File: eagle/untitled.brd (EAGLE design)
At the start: 56.8 x 71.1 mm, 30 parts, among them IC1 74HC595D, IC2 74HC595D, Q1 BC557, Q2 BC557, Q3 BC557, Q4 BC557, Q5 BC557, Q6 BC547, Q7 BC547, Q8 BC547

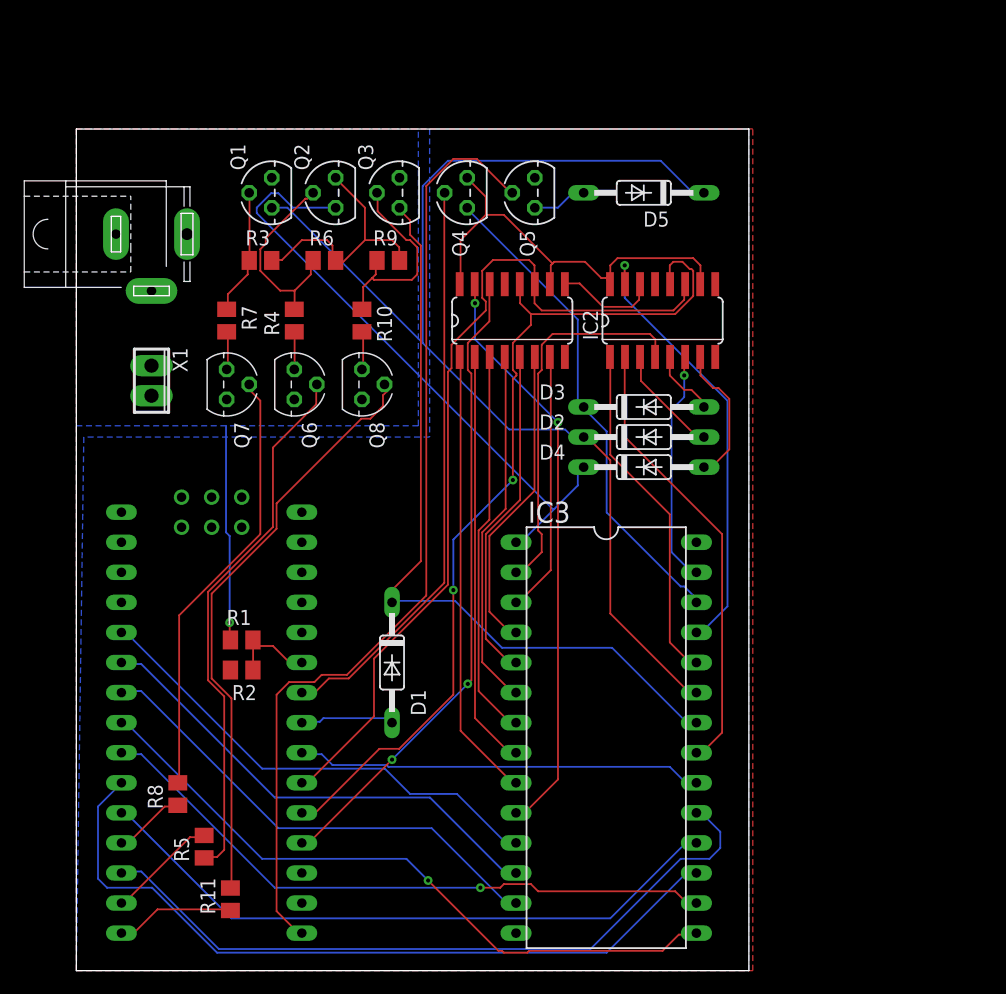
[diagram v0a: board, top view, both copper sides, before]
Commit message: Исправления схемы.
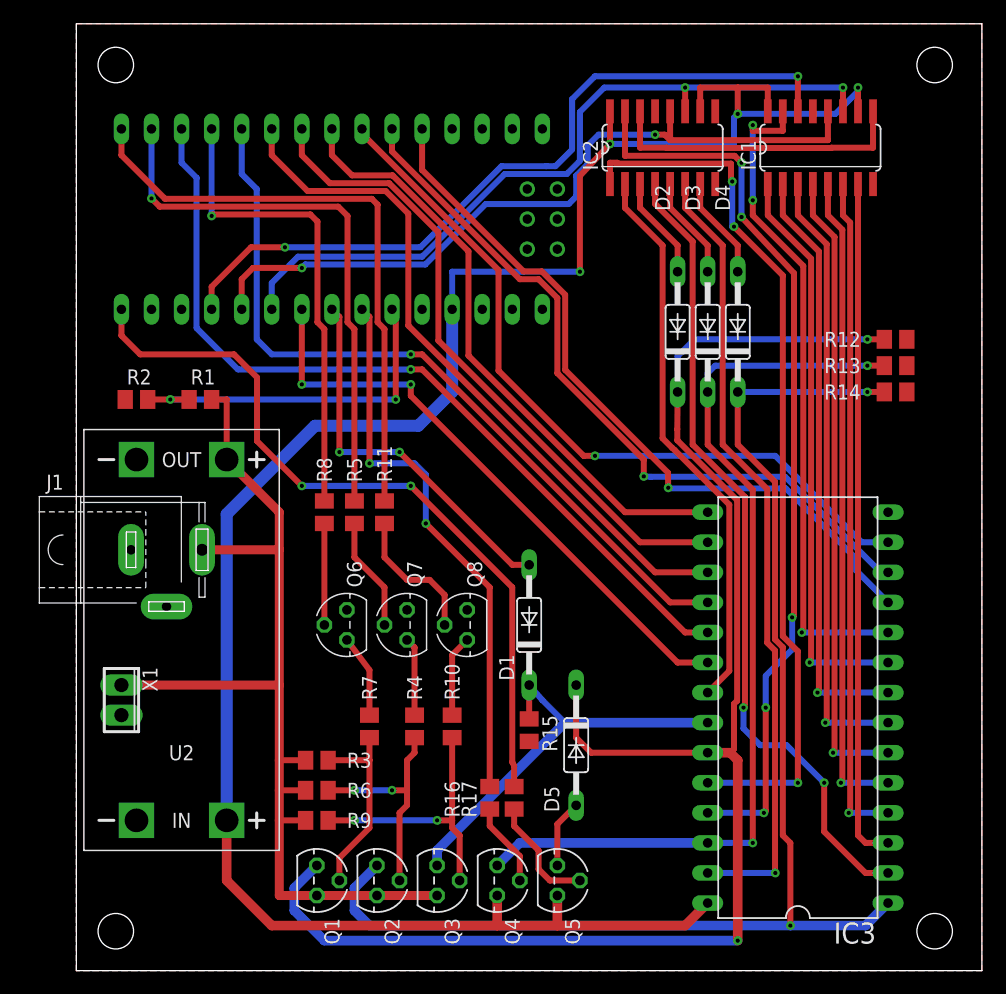
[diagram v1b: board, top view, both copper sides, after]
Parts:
- removed U$1: NANO, Arduino-clone:NANO
- added R12, R13, R14, R15: 4.7K, rcl:M0805
- added R16, R17: 300, rcl:M0805
- added U1: NANO, Arduino-clone:NANO
- added U2: DC-DC-STEP-UP-MT3608, diy-modules:DC-DC-STEP-UP-MT3608
- moved Q1 58.2 mm to (20.3, 7.62), turned to 270 degrees
- moved Q2 58.2 mm to (25.4, 7.62), turned to 270 degrees
- moved Q3 58.2 mm to (30.5, 7.62), turned to 270 degrees
- moved Q4 58.2 mm to (35.6, 7.62), turned to 270 degrees
- moved Q5 58.1 mm to (40.6, 7.62), turned to 270 degrees
- moved R9 47.7 mm to (20.3, 12.7), turned to 180 degrees
- moved D5 47.0 mm to (42.2, 19.1), turned to 270 degrees
- moved R6 44.8 mm to (20.3, 15.2), turned to 180 degrees
- moved R3 42.5 mm to (20.3, 17.8), turned to 180 degrees
- moved R7 36.4 mm to (24.8, 20.6), turned to 90 degrees
- moved R4 35.8 mm to (28.6, 20.6), turned to 270 degrees
- moved R11 35.2 mm to (26.0, 38.7), turned to 270 degrees
- moved R10 35.1 mm to (31.8, 20.6), turned to 90 degrees
- moved R5 31.0 mm to (23.5, 38.7)
- moved IC1 29.9 mm to (62.9, 69.5)
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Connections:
- new net N$25: Q4.2, R16.2
- new net N$26: Q5.2, R17.2
- net +24V: now also U2.OUT+
- net A11: now also R12.1
- net A13: now also R13.1
- net A15: now also R14.1
- net CE: now also U1.A3; no longer U$1.A3
- net D0: now also U1.D2; no longer U$1.D2
- net D1: now also U1.D3; no longer U$1.D3
- net D2: now also U1.D4; no longer U$1.D4
- net D3: now also U1.D5; no longer U$1.D5
- net D4: now also U1.D6; no longer U$1.D6
- net D5: now also U1.D7; no longer U$1.D7
- net D6: now also U1.D8; no longer U$1.D8
- net D7: now also U1.D10; no longer U$1.D10
- net GND: now also R12.2, R13.2, R14.2, R15.2, U1.GND, U1.GND1, U2.IN-, U2.OUT-; no longer U$1.GND
- net N$1: now also U1.A2; no longer U$1.A2
- net N$10: now also R16.1, U1.A5; no longer Q4.2, U$1.A5
- net N$11: now also U1.D11; no longer U$1.D11
- net N$12: now also R17.1, U1.D13; no longer Q5.2, U$1.D13
- net N$13: now also U1.D12; no longer U$1.D12
- net N$19: now also Q7.3; no longer Q6.3
- net N$2: now also U1.A1; no longer U$1.A1
- net N$21: now also Q7.2; no longer Q6.2
- net N$22: now also Q6.3; no longer Q7.3
- net N$24: now also Q6.2; no longer Q7.2
- net N$4: now also U1.A0; no longer U$1.A0
- net N$7: now also U1.D9; no longer U$1.D9
- net N$8: now also U1.A4; no longer U$1.A4
- net N$9: now also U1.A6; no longer U$1.A6
- net OE: now also R15.1
- net VCC: now also U1.5V, U2.IN+; no longer U$1.5V
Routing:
- net VCC: track 37.1 -> 176.3 mm, vias 0 -> 4
- net A15: track 52.6 -> 110.3 mm, vias 0 -> 2
- net A14: track 19.8 -> 67.1 mm
- net +24V: track 39.5 -> 84.9 mm, vias 1 -> 0
- net A9: track 29.2 -> 74.5 mm, vias 0 -> 3
- net N$13: track 10.1 -> 50.9 mm
- net A8: track 37.6 -> 76.3 mm, vias 1 -> 5
- net N$18: track 50.0 -> 11.8 mm
- net N$11: track 9.40 -> 47.4 mm, vias 0 -> 1
- net A13: track 41.5 -> 78.8 mm, vias 0 -> 2
- net A12: track 32.3 -> 68.9 mm, vias 0 -> 2
- net N$21: track 45.7 -> 9.63 mm
- net A7: track 22.2 -> 57.8 mm
- net N$7: track 6.12 -> 40.4 mm, vias 0 -> 1
- net A11: track 99.5 -> 131.1 mm, vias 0 -> 2
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- removed copper zone on layer 16, net +24V
- removed copper zone on layer 16, net VCC
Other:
- board size 56.8 x 71.1 mm -> 76.5 x 80 mm
